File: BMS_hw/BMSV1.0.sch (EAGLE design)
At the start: 225 parts, among them IC1 MC33771BEP, IC2 SFH6156, IC3 MIC28515V1, IC4 FOD8384-COC, IC5 FOD8384-COC, IC6 FOD8384-COC, J2 NTC, Q1 IRLML5203, Q2 IRLML5203, T1 IPT020N10N3V1, T2 IPT020N10N3V1, T3 IPT020N10N3V1, T4 IPT020N10N3V1, X1 87758-2016, X2 87758-1816, X4 87758-2016

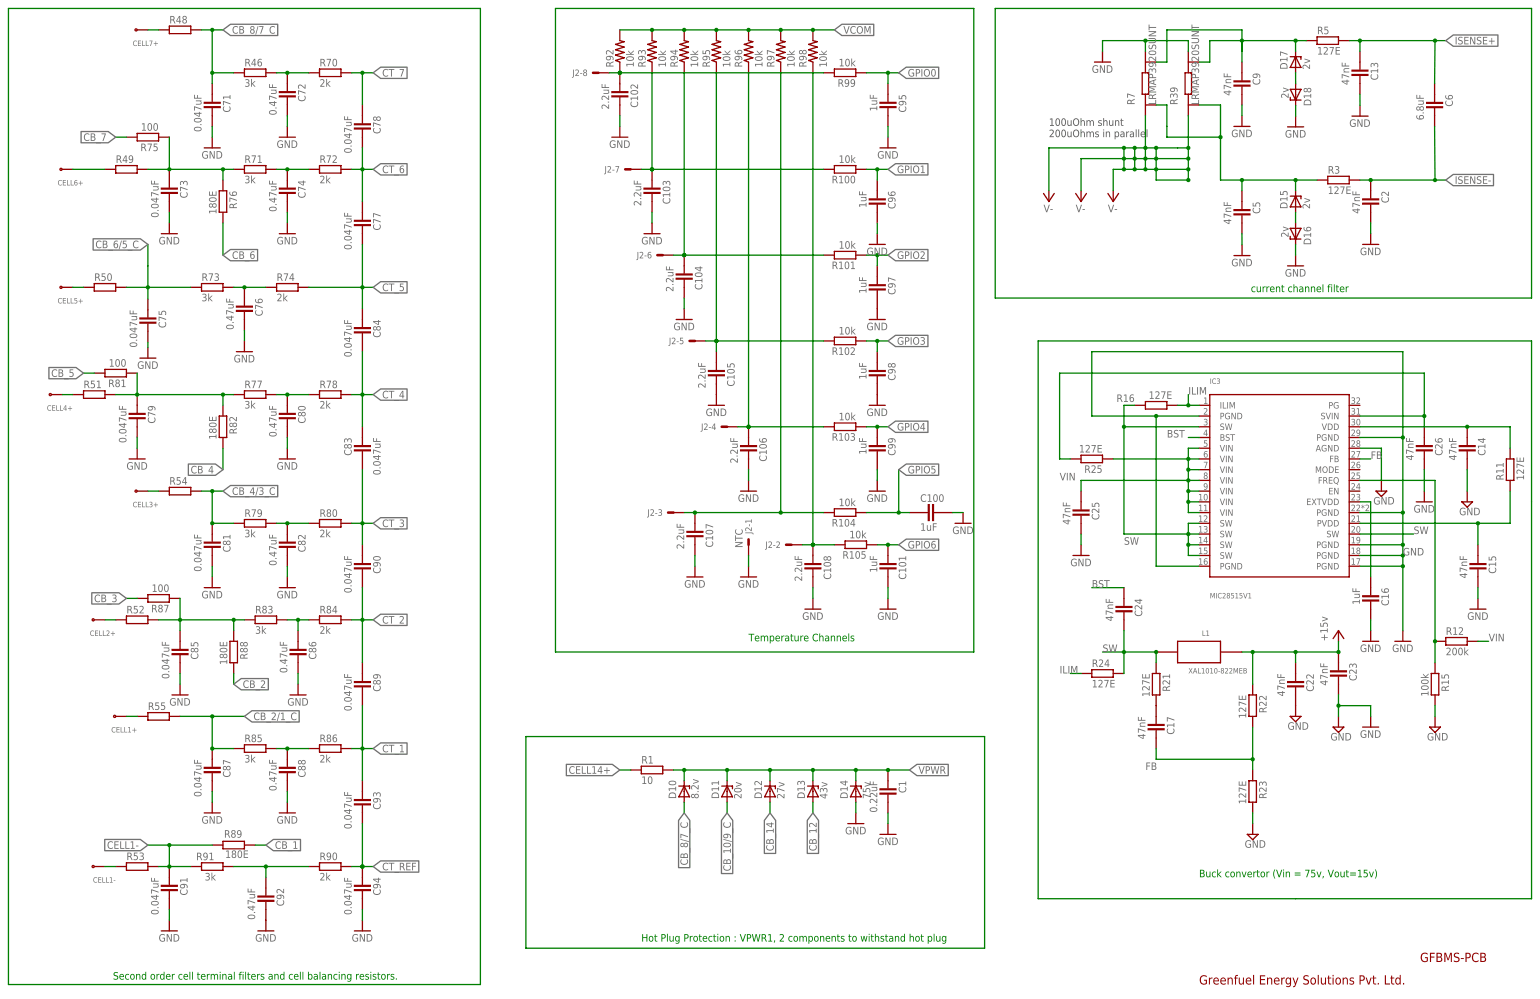
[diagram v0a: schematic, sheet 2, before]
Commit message: brd lbr sch updated to new version
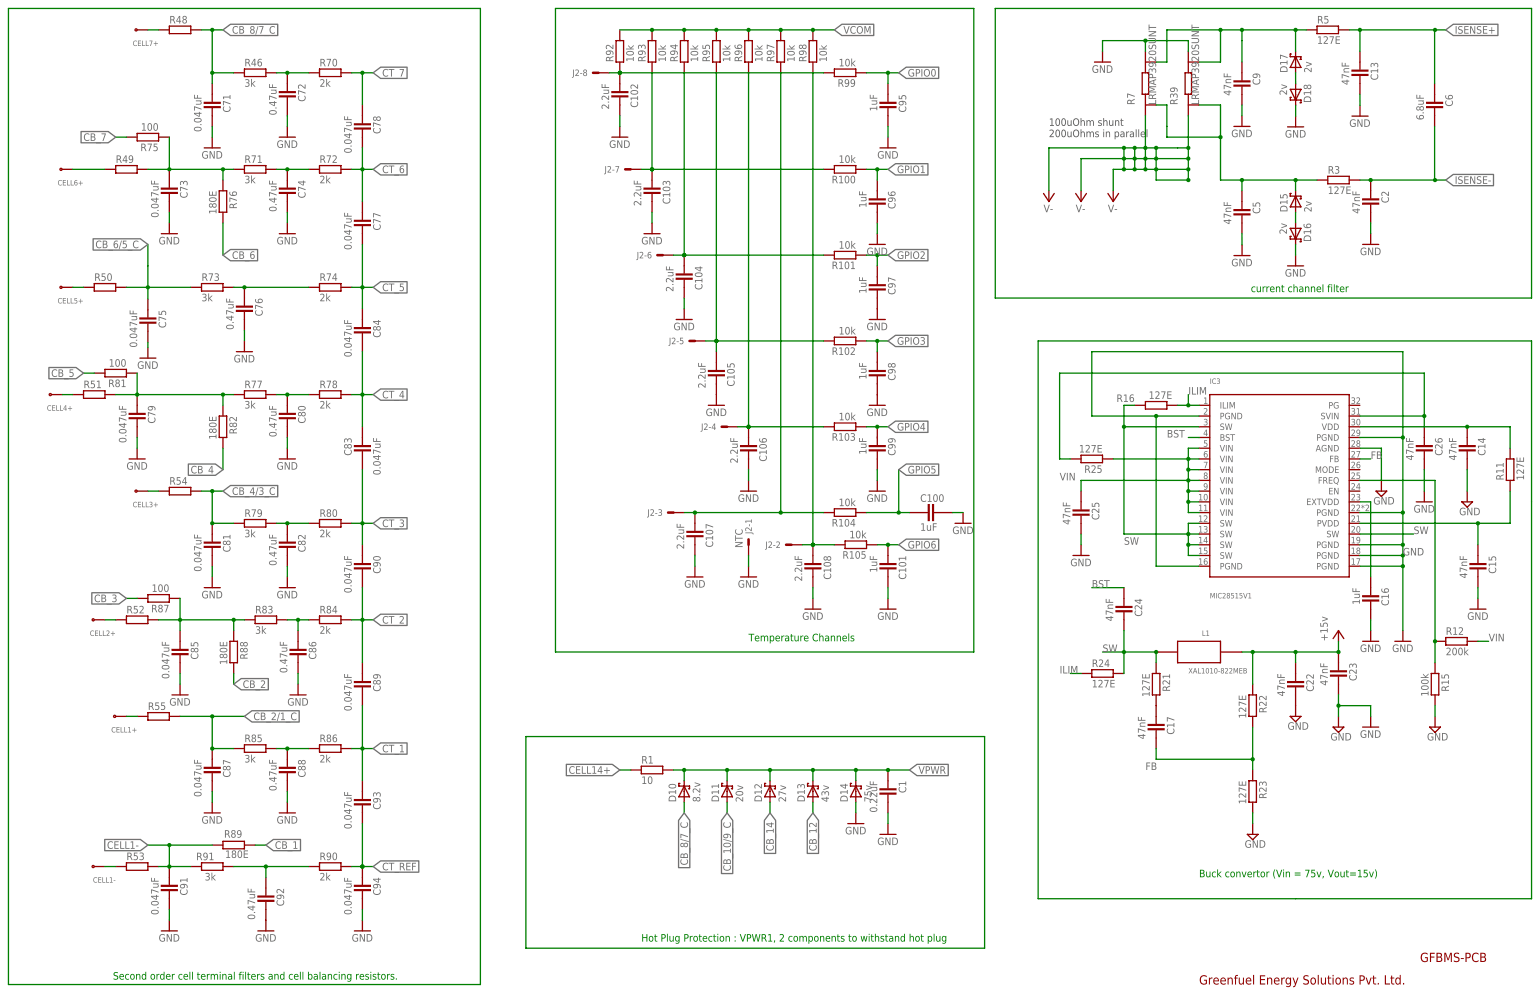
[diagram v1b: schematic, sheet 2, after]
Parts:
- D10, D11, D12, D13, D14, D15, D16, D17, D18: device diode:ZENER-DIODESOD80C -> ipc-7351-diode:SCHOTTKY_SOD-123
- R92, R93, R94, R95, R96, R97, R98: device adafruit:R-US_R0805 -> ipc-7351-resistor:RESISTOR_0402
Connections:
- removed net N$15: D17.C, R5.1
- net GND: now also D16.K, D18.K; no longer D16.C, D18.C
- net N$68: now also D17.K, R5.1
- net N$70: now also D15.K; no longer D15.C
- net VPWR: now also D10.K, D11.K, D12.K, D13.K, D14.K; no longer D10.C, D11.C, D12.C, D13.C, D14.C
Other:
- moved on the sheet: R5, R74
